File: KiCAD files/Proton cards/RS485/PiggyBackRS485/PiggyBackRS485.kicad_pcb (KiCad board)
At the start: 2 copper layers, 35.1 x 35.1 mm, 10 parts, among them J1 RS485 (net0), J2 terminal, J3 Conn_01x08, J4 RS485 (net1), J5 terminal, U1 SN75176AP, U2 SN75176AP

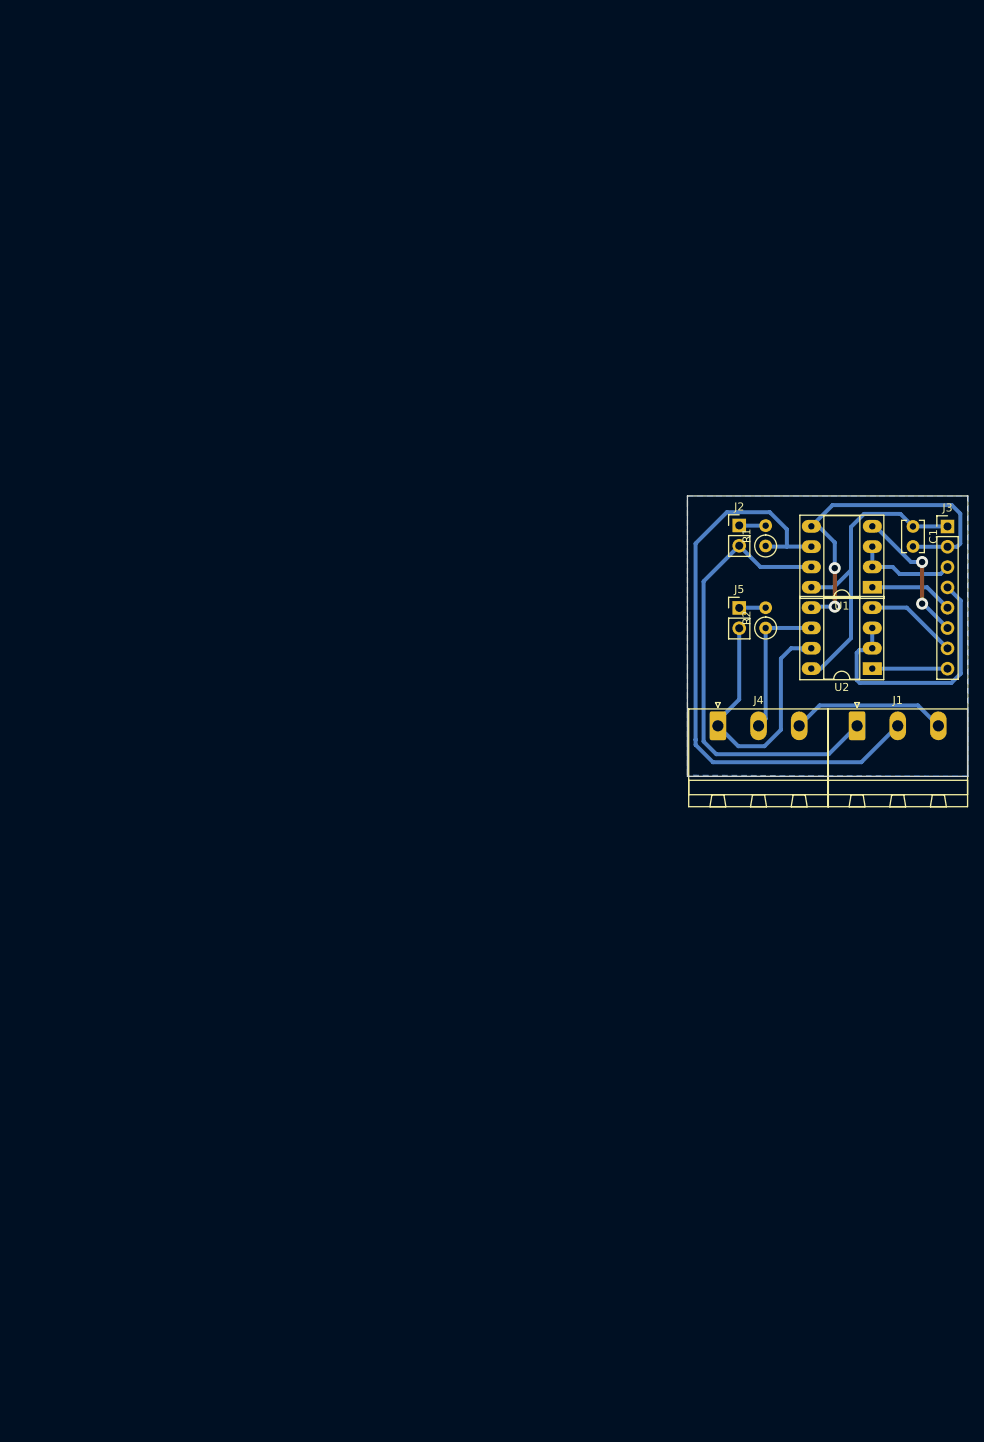
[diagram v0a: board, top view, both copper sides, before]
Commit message: pcbs
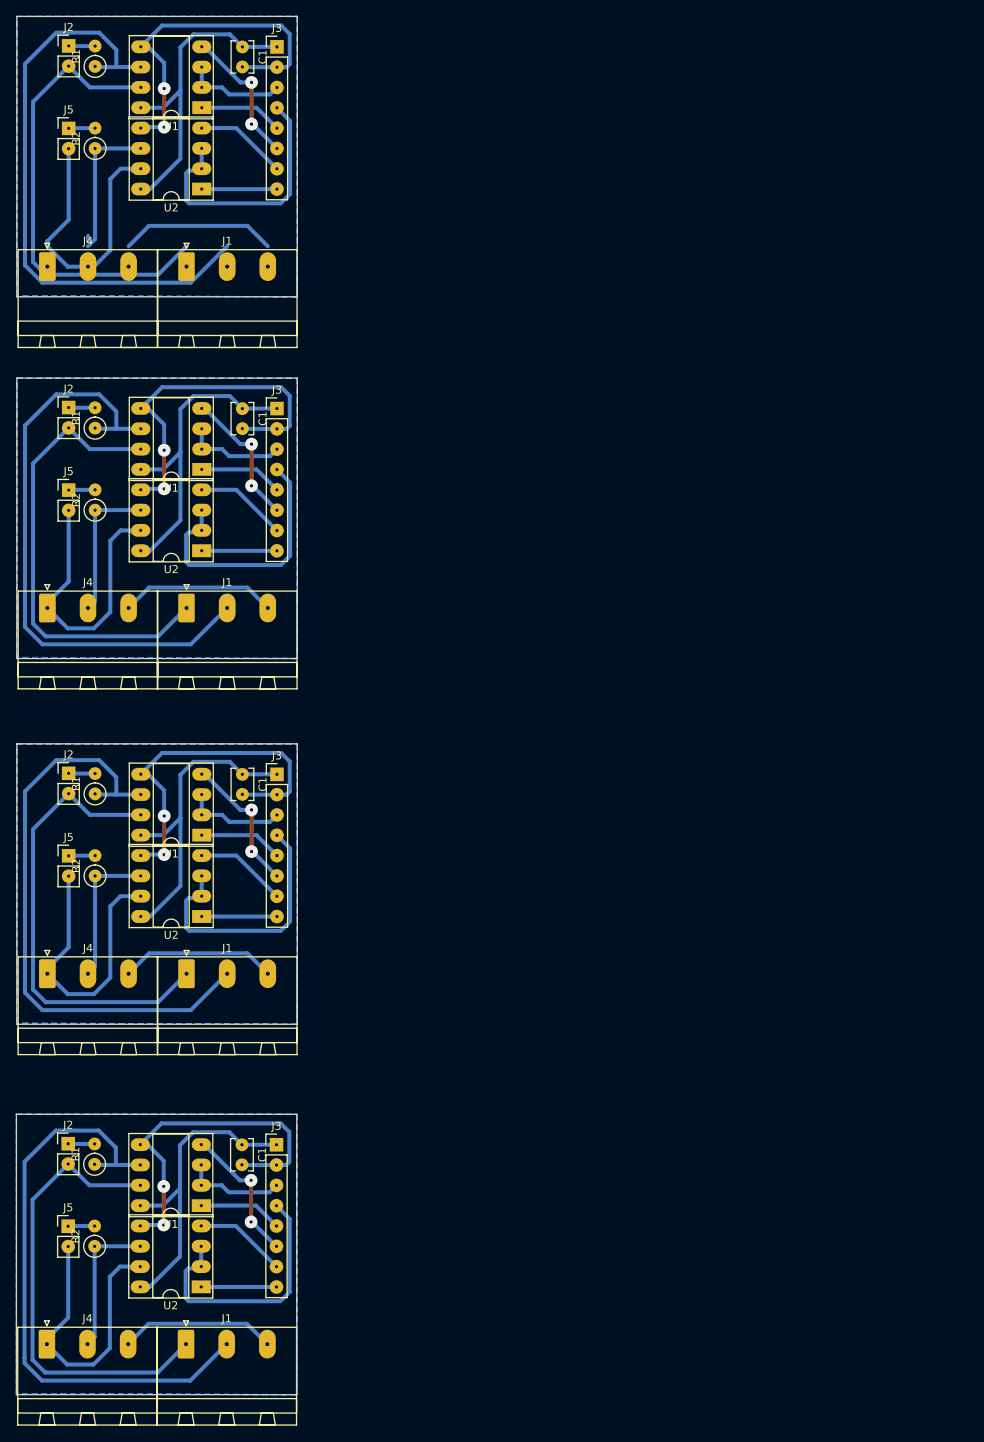
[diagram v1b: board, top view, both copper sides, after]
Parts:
- added C1: 100nF, Capacitor_THT:C_Disc_D3.8mm_W2.6mm_P2.50mm, F.Cu at (46.5, 19.6)
- added C1: 100nF, Capacitor_THT:C_Disc_D3.8mm_W2.6mm_P2.50mm, F.Cu at (46.4, 156.8)
- added C1: 100nF, Capacitor_THT:C_Disc_D3.8mm_W2.6mm_P2.50mm, F.Cu at (46.5, 110.5)
- added J1: RS485 (net0), Connector_Phoenix_MSTB:PhoenixContact_MSTBA_2,5_3-G-5,08_1x03_P5.08mm_Horizontal, F.Cu at (39.4, 181.7)
- added J1: RS485 (net0), Connector_Phoenix_MSTB:PhoenixContact_MSTBA_2,5_3-G-5,08_1x03_P5.08mm_Horizontal, F.Cu at (39.5, 47.0)
- added J1: RS485 (net0), Connector_Phoenix_MSTB:PhoenixContact_MSTBA_2,5_3-G-5,08_1x03_P5.08mm_Horizontal, F.Cu at (39.5, 135.4)
- added J2: terminal, Connector_PinHeader_2.54mm:PinHeader_1x02_P2.54mm_Vertical, F.Cu at (24.8, 19.4)
- added J2: terminal, Connector_PinHeader_2.54mm:PinHeader_1x02_P2.54mm_Vertical, F.Cu at (24.7, 156.7)
- added J2: terminal, Connector_PinHeader_2.54mm:PinHeader_1x02_P2.54mm_Vertical, F.Cu at (24.8, 110.4)
- added J3: Conn_01x08, Connector_PinHeader_2.54mm:PinHeader_1x08_P2.54mm_Vertical, F.Cu at (50.7, 156.8)
- added J3: Conn_01x08, Connector_PinHeader_2.54mm:PinHeader_1x08_P2.54mm_Vertical, F.Cu at (50.8, 19.6)
- added J3: Conn_01x08, Connector_PinHeader_2.54mm:PinHeader_1x08_P2.54mm_Vertical, F.Cu at (50.8, 110.5)
- added J4: RS485 (net1), Connector_Phoenix_MSTB:PhoenixContact_MSTBA_2,5_3-G-5,08_1x03_P5.08mm_Horizontal, F.Cu at (22.1, 47.0)
- added J4: RS485 (net1), Connector_Phoenix_MSTB:PhoenixContact_MSTBA_2,5_3-G-5,08_1x03_P5.08mm_Horizontal, F.Cu at (22.0, 181.7)
- added J4: RS485 (net1), Connector_Phoenix_MSTB:PhoenixContact_MSTBA_2,5_3-G-5,08_1x03_P5.08mm_Horizontal, F.Cu at (22.1, 135.4)
- added J5: terminal, Connector_PinHeader_2.54mm:PinHeader_1x02_P2.54mm_Vertical, F.Cu at (24.7, 167.0)
- added J5: terminal, Connector_PinHeader_2.54mm:PinHeader_1x02_P2.54mm_Vertical, F.Cu at (24.8, 29.7)
- added J5: terminal, Connector_PinHeader_2.54mm:PinHeader_1x02_P2.54mm_Vertical, F.Cu at (24.8, 120.7)
- added R1: 150, Resistor_THT:R_Axial_DIN0207_L6.3mm_D2.5mm_P2.54mm_Vertical, F.Cu at (28.0, 159.2)
- added R1: 150, Resistor_THT:R_Axial_DIN0207_L6.3mm_D2.5mm_P2.54mm_Vertical, F.Cu at (28.1, 22.0)
- added R1: 150, Resistor_THT:R_Axial_DIN0207_L6.3mm_D2.5mm_P2.54mm_Vertical, F.Cu at (28.1, 112.9)
- added R2: 150, Resistor_THT:R_Axial_DIN0207_L6.3mm_D2.5mm_P2.54mm_Vertical, F.Cu at (28.0, 169.5)
- added R2: 150, Resistor_THT:R_Axial_DIN0207_L6.3mm_D2.5mm_P2.54mm_Vertical, F.Cu at (28.1, 32.3)
- added R2: 150, Resistor_THT:R_Axial_DIN0207_L6.3mm_D2.5mm_P2.54mm_Vertical, F.Cu at (28.1, 123.2)
- added U1: SN75176AP, Package_DIP:DIP-8_W7.62mm_Socket_LongPads, F.Cu at (41.4, 27.2)
- added U1: SN75176AP, Package_DIP:DIP-8_W7.62mm_Socket_LongPads, F.Cu at (41.3, 164.4)
- added U1: SN75176AP, Package_DIP:DIP-8_W7.62mm_Socket_LongPads, F.Cu at (41.4, 118.1)
- added U2: SN75176AP, Package_DIP:DIP-8_W7.62mm_Socket_LongPads, F.Cu at (41.4, 128.3)
- added U2: SN75176AP, Package_DIP:DIP-8_W7.62mm_Socket_LongPads, F.Cu at (41.3, 174.6)
- added U2: SN75176AP, Package_DIP:DIP-8_W7.62mm_Socket_LongPads, F.Cu at (41.4, 37.3)
- moved J3 85.1 mm to (50.8, 64.8)
- moved J4 85.1 mm to (22.1, 89.7)
- moved C1 85.1 mm to (46.5, 64.8)
- moved J1 85.1 mm to (39.5, 89.7)
- moved J2 85.1 mm to (24.8, 64.6)
- moved J5 85.1 mm to (24.8, 75.0)
- moved R1 85.1 mm to (28.1, 67.2)
- moved R2 85.1 mm to (28.1, 77.5)
- moved U1 85.1 mm to (41.4, 72.4)
- moved U2 85.1 mm to (41.4, 82.5)
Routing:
- net Net-(J1-Pad2): track 75.1 -> 300.2 mm
- net Net-(J1-Pad1): track 57.8 -> 231.0 mm
- net GND: track 44.9 -> 179.6 mm, vias 2 -> 8
- net +5V: track 40.6 -> 162.5 mm
- net Net-(J4-Pad1): track 37.1 -> 148.5 mm
- net /DE1: track 33.1 -> 132.4 mm
- net Earth_Protective: track 19.5 -> 78.0 mm
- net Net-(J4-Pad2): track 18.8 -> 75.3 mm
- net /TX0: track 17.7 -> 70.9 mm, vias 2 -> 8
- net /DE0: track 13.7 -> 54.9 mm
- net /TX1: track 11.5 -> 46.1 mm
- net /RX0: track 10.5 -> 41.8 mm
- net /RX1: track 9.74 -> 38.9 mm
- net Net-(J2-Pad1): track 3.31 -> 13.3 mm
- net Net-(J5-Pad1): track 3.31 -> 13.3 mm
- added copper zone on B.Cu, net GND
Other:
- board size 35.1 x 35.1 mm -> 35.1 x 172.3 mm
